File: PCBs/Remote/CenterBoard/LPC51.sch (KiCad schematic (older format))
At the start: 25 parts, among them J201 DX07S016JA1R1500, U201 LPC51U68JBD64

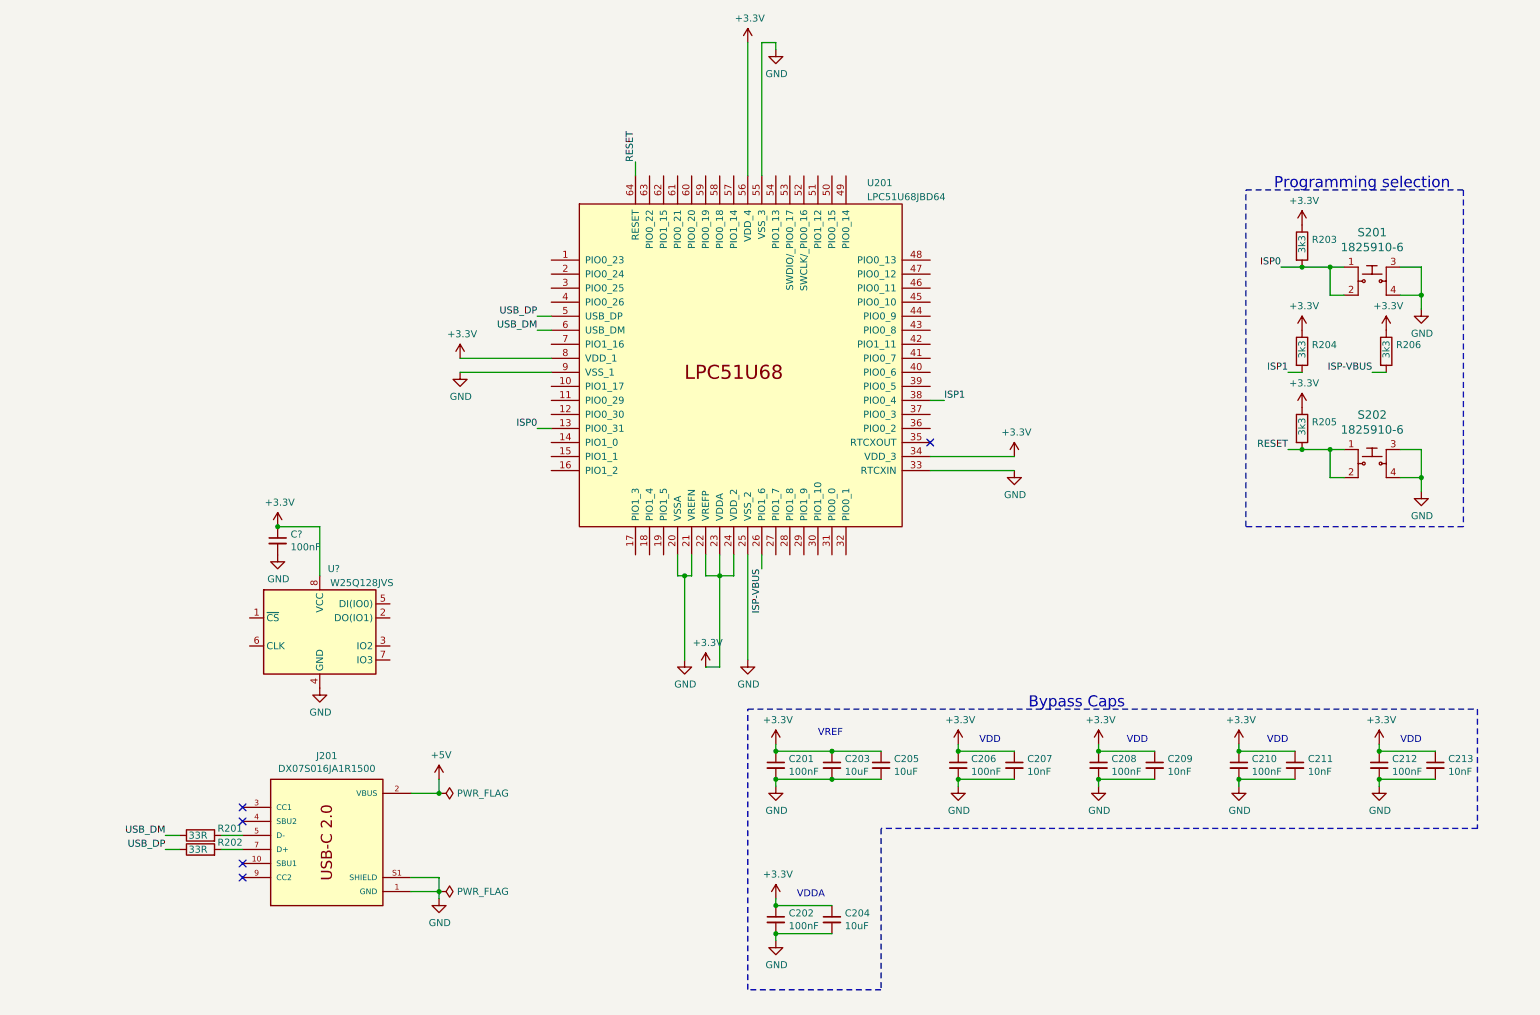
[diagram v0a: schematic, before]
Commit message: Continued work with the center board
Signed-off-by: Eldalote.Electronics <Eldalote.Electronics@gmail.com>
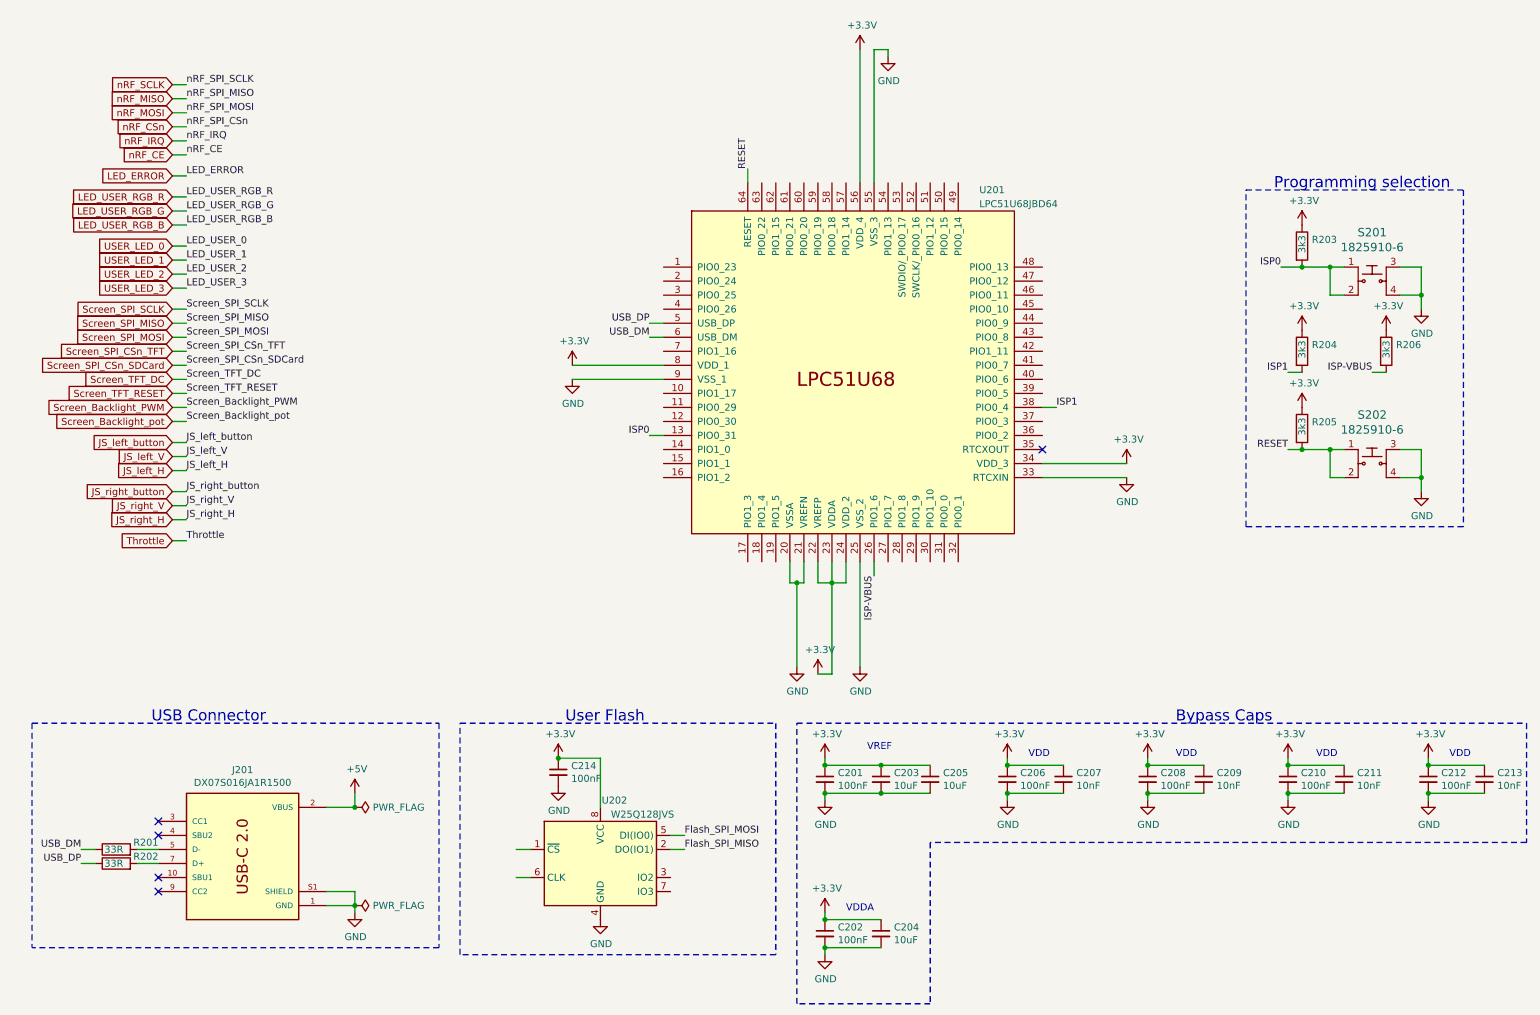
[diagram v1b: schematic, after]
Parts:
- U201: DigiKey (none) -> 568-13909-ND; Mouser (none) -> 771-LPC51U68JBD64QL
- U202: renamed from U?; LCSC (none) -> C97521
- gave numbers to parts that had none: 1
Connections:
- net Flash_SPI_MISO: now reaches U202.2 (DO(IO1))
- net Flash_SPI_MOSI: now reaches U202.5 (DI(IO0))
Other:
- note added: "USB Connector"
- note added: "User Flash"
- moved on the sheet: C201, C202, C203, C204, C205, C206, C207, C208, C209, C210, C211, C212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
